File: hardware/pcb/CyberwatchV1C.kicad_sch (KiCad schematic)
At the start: 6 parts, among them J1 MEM2080-00-128-00-A_REVA, U1 ESP32-S3-WROOM-1, U2 RV-3028-C7, U3 MAX17048G_T10

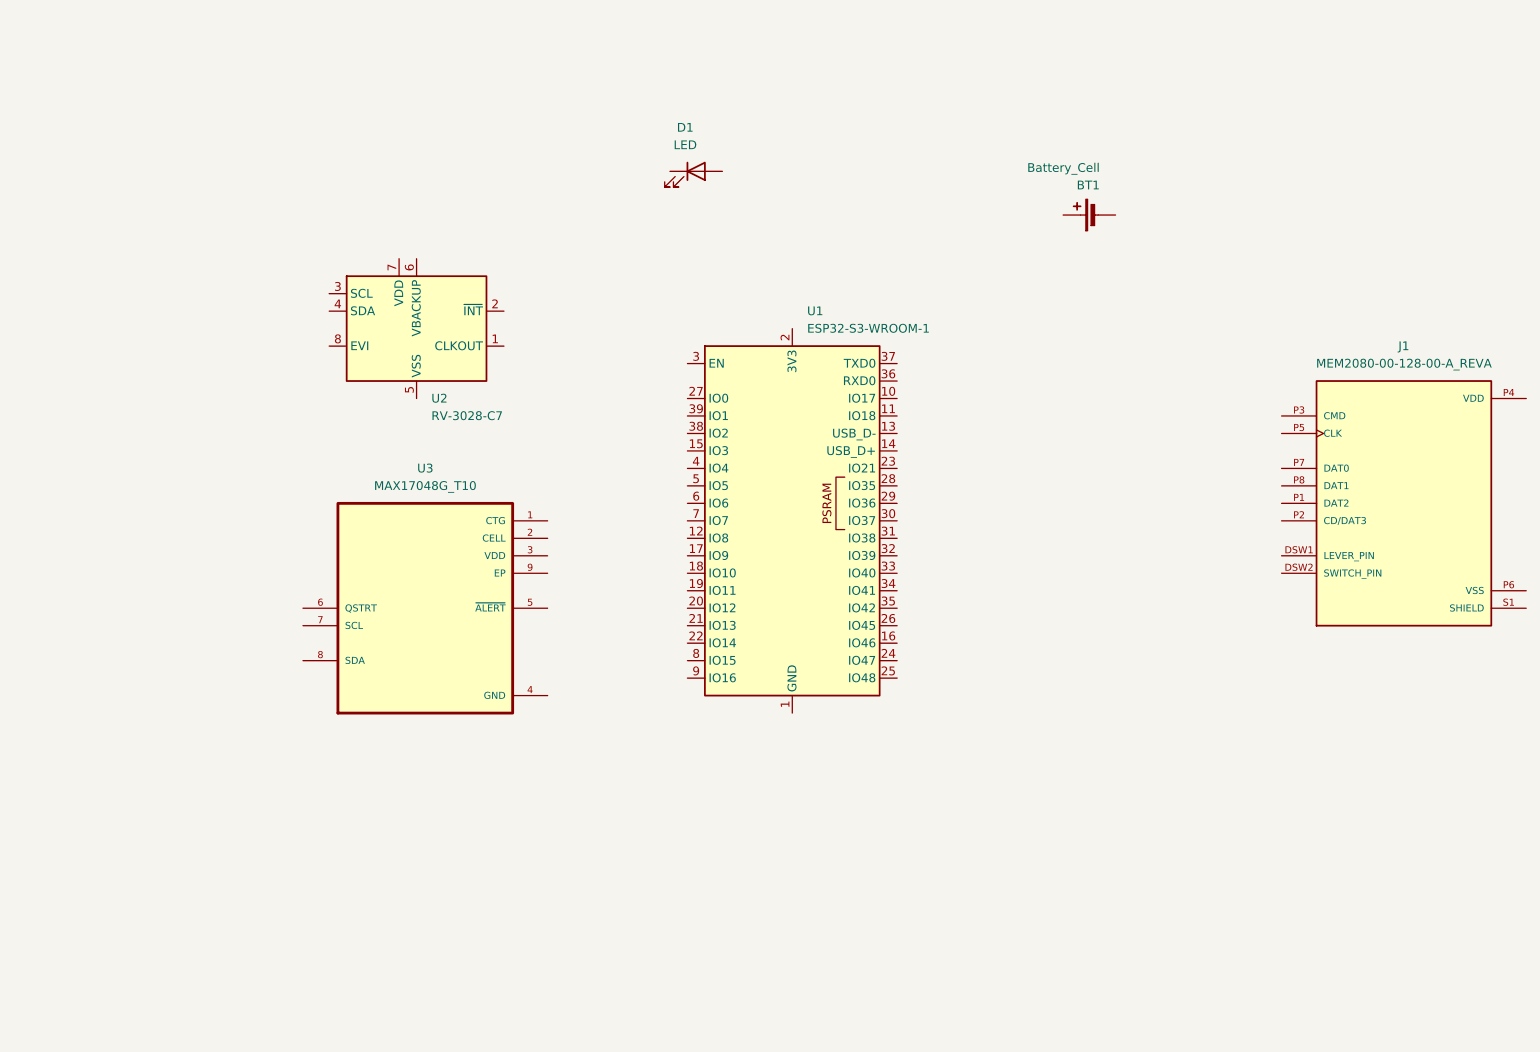
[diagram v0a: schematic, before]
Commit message: schematic progress
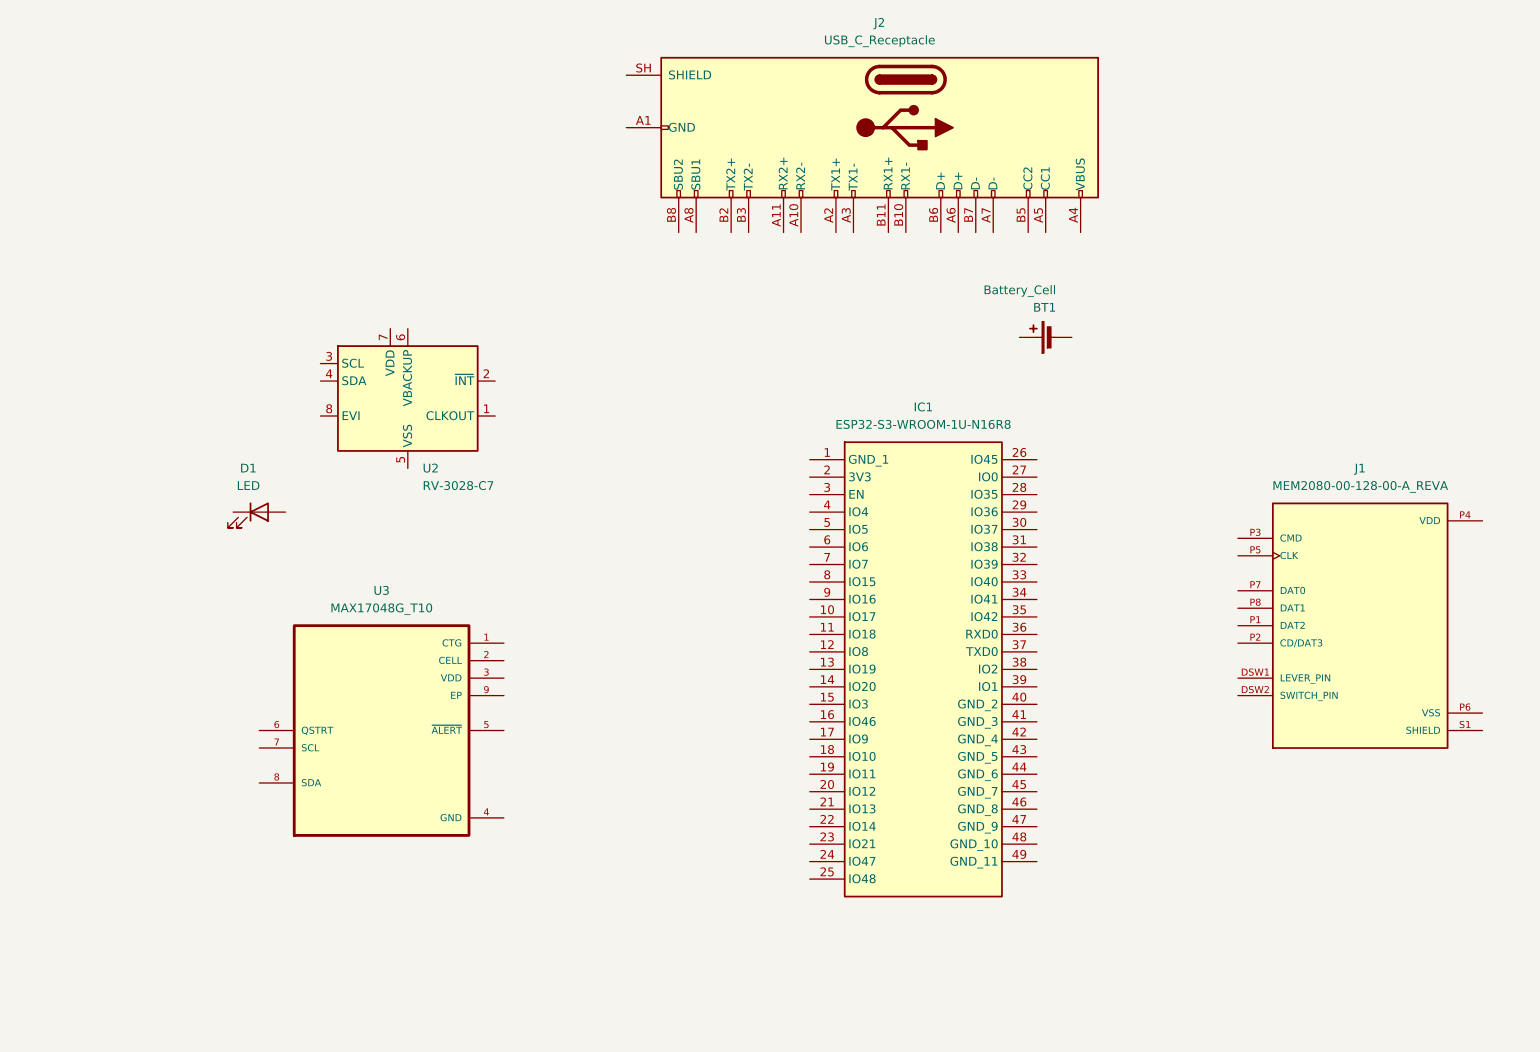
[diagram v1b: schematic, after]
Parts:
- removed U1: ESP32-S3-WROOM-1, RF_Module:ESP32-S3-WROOM-1, symbol RF_Module:ESP32-S3-WROOM-1
- added IC1: ESP32-S3-WROOM-1U-N16R8, RF_Module:ESP32-S3-WROOM-1U, symbol ESP32-S3:ESP32-S3-WROOM-1U-N16R8
- added J2: USB_C_Receptacle, symbol Connector:USB_C_Receptacle
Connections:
- new net: J2.A1 (GND), J2.A12 (GND), J2.B1 (GND), J2.B12 (GND)
- new net: J2.A4 (VBUS), J2.A9 (VBUS), J2.B4 (VBUS), J2.B9 (VBUS)
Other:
- moved on the sheet: BT1, D1, J1, U2, U3

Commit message: schematic progress
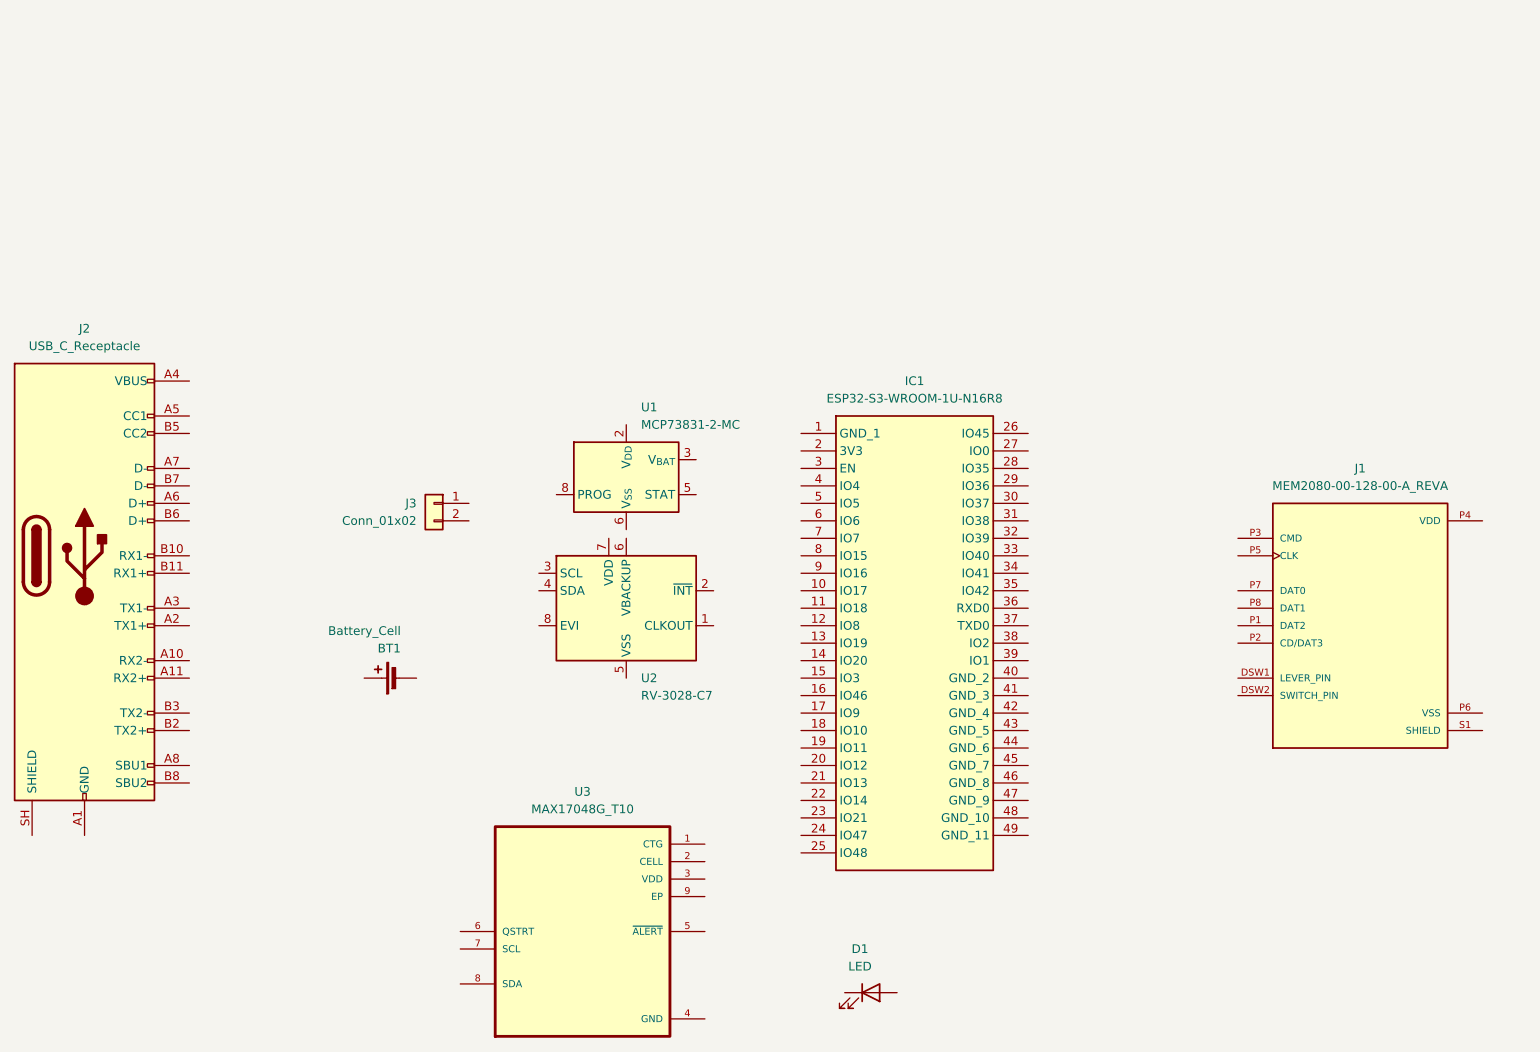
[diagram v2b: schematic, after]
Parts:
- added J3: Conn_01x02, symbol Connector_Generic:Conn_01x02
- added U1: MCP73831-2-MC, Package_DFN_QFN:DFN-8-1EP_3x2mm_P0.5mm_EP1.7x1.4mm, symbol Battery_Management:MCP73831-2-MC
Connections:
- new net: U1.1 (V_{DD}), U1.2 (V_{DD})
- new net: U1.3 (V_{BAT}), U1.4 (V_{BAT})
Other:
- moved on the sheet: BT1, D1, IC1, J2, U2, U3
